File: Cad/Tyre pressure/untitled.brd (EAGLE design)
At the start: 160 x 100 mm, 13 parts, among them IC1 MCP1703CB

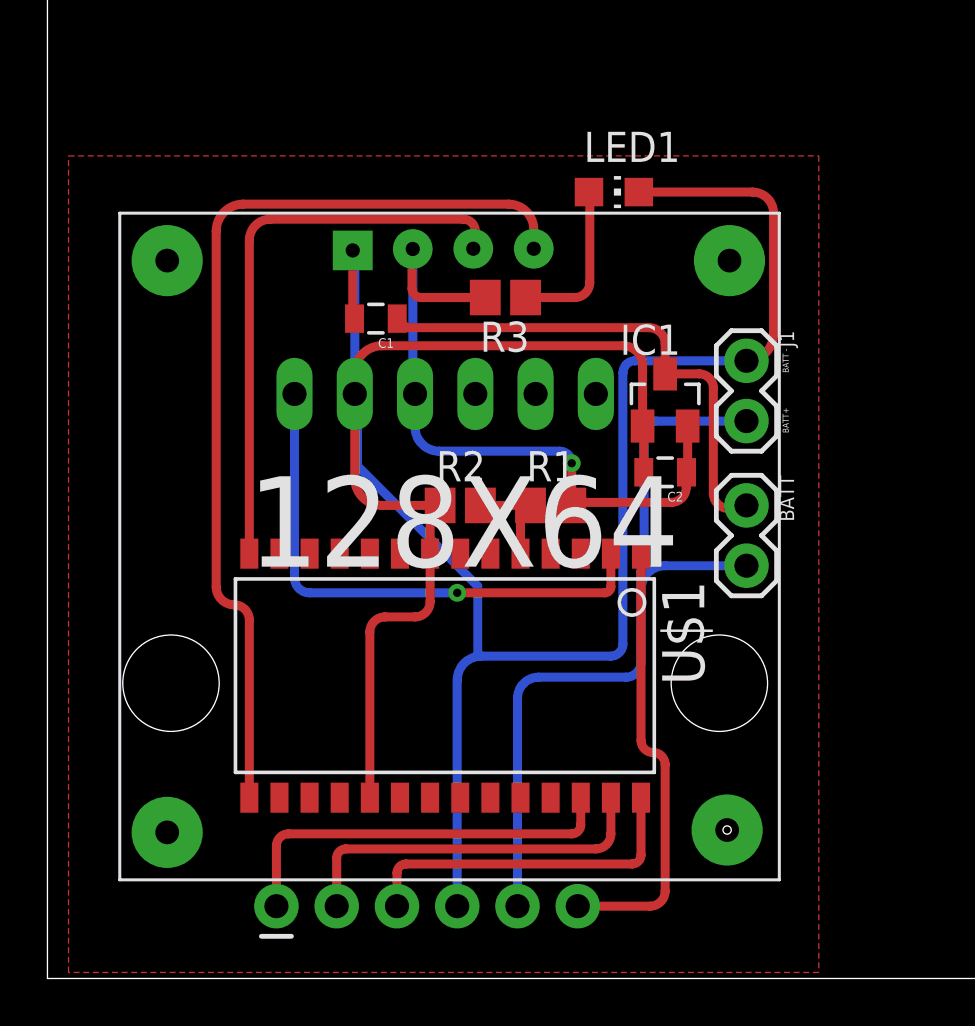
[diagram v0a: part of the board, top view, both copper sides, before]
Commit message: add gerber
Add gerber and layout to the board
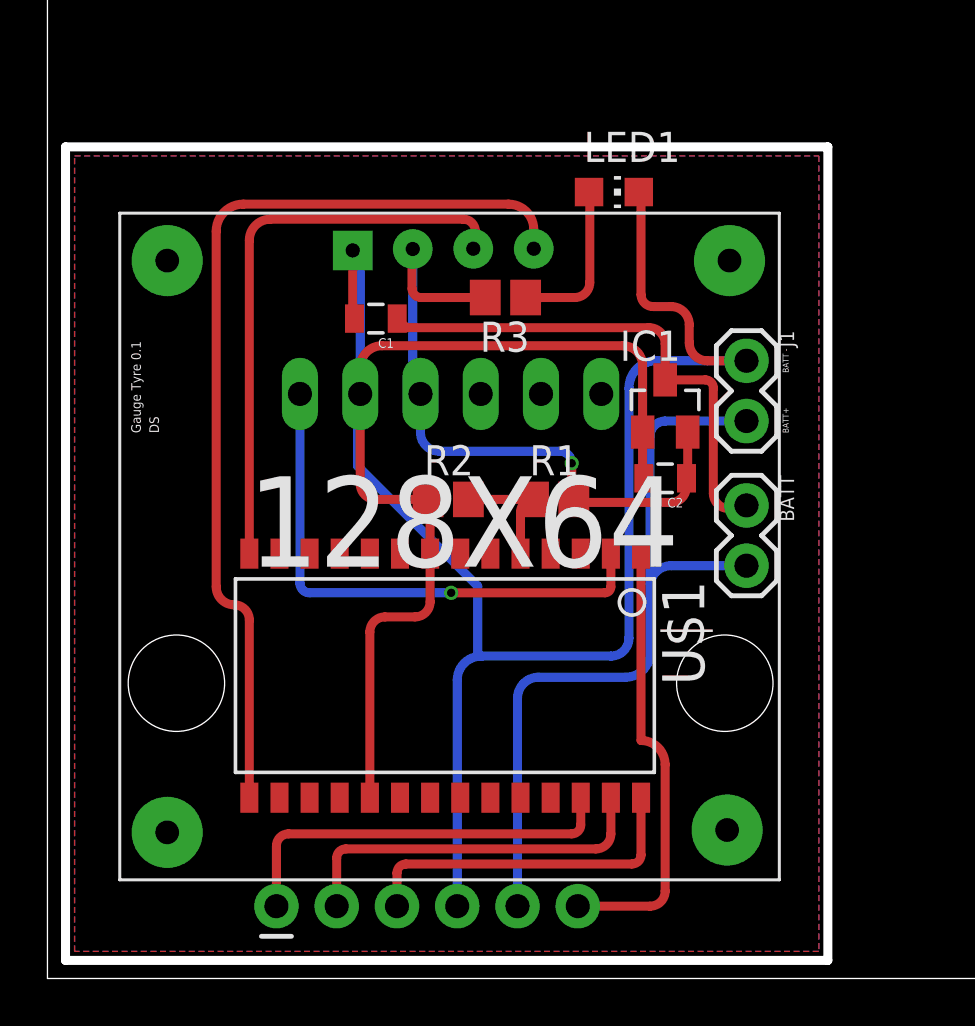
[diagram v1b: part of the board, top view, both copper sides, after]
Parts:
- moved R2 0.57 mm to (16.9, 20.2)
- moved R1 0.28 mm to (21.3, 20.2)
- moved IC1 0.25 mm to (26.0, 24.1)
- moved C2 0.25 mm to (26.0, 21.1)
- moved PS1 0.23 mm to (17.0, 12.4)
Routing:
- net GND: track 109.8 -> 106.8 mm
- net 3V: track 4.32 -> 5.26 mm
- net VCC: track 33.7 -> 33.0 mm
- added copper zone on layer 16, net BOTTOMPOLY
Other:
- outline, holes or cut-outs redrawn
- board text added: "DS"
- board text added: "Gauge Tyre 0.1"
